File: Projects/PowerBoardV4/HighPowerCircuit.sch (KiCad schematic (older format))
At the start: 27 parts, among them J1 Cell Voltage Sense, J10 5V_INT_PWR_BLK, J11 5V_INT_PWR_BLK, J12 5V_INT_PWR_BLK, J13 5V_INT_PWR_BLK, J14 12V_INT_PWR_BLK, J15 12V_INT_PWR_BLK, J16 12V_INT_PWR_BLK, J17 12V_INT_PWR_BLK, J2 BATT_PWR, J3 12V POWER SUPPLY, J4 5V POWER SUPPLY, J5 BACK_EXT_24V, J7 MC_STACK_1, J8 MC_STACK_2, J9 24V_INT_PWR_BLK, Q1 IRF3205, Q2 IRF3205, Q3 BSS84

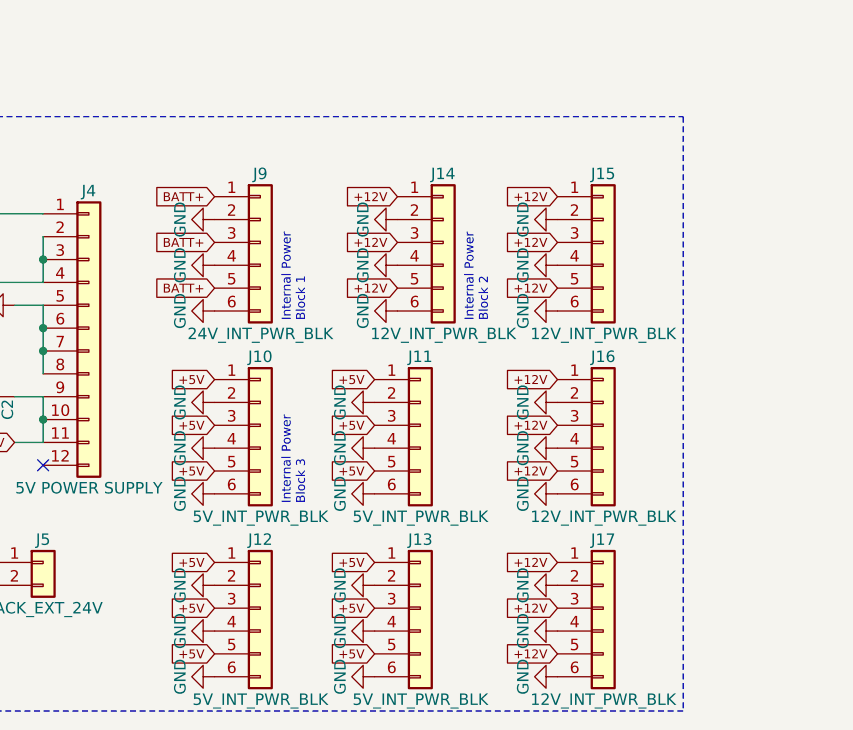
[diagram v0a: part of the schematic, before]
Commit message: Changes complete and ready for review
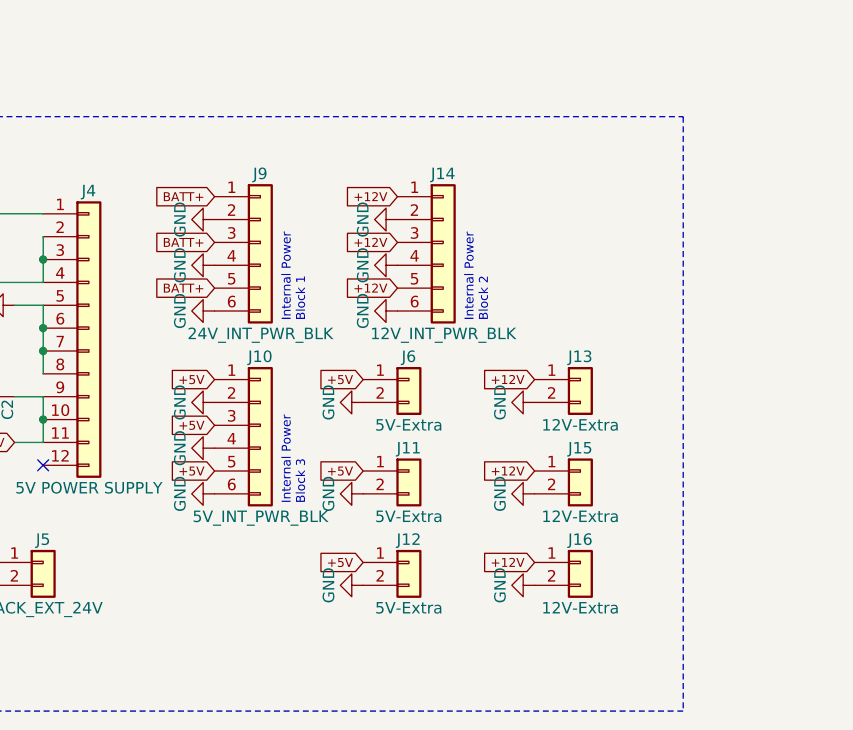
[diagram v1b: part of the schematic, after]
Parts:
- removed J11, J12, J13: 5V_INT_PWR_BLK, Terminal_Blocks:TerminalBlock_Pheonix_PT-3.5mm_6pol, symbol Conn_01x06
- removed J15, J16, J17: 12V_INT_PWR_BLK, USST-footprints:TerminalBlock_Pheonix_PT-5mm_6pol, symbol Conn_01x06
- added J11, J12, J6: 5V-Extra, USST-footprints:Molex_39531_1002, symbol Conn_01x02
- added J13, J15, J16: 12V-Extra, USST-footprints:Molex_39531_1002, symbol Conn_01x02
- J14: footprint USST-footprints:TerminalBlock_Pheonix_PT-5mm_6pol -> Terminal_Blocks:TerminalBlock_Pheonix_PT-3.5mm_6pol
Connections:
- net +12V: now also J13.1 (Pin_1), J15.1 (Pin_1), J16.1 (Pin_1)
- net +5V: now also J11.1 (Pin_1), J12.1 (Pin_1), J6.1 (Pin_1)
- net GND: now also J11.2 (Pin_2), J12.2 (Pin_2), J13.2 (Pin_2), J15.2 (Pin_2), J16.2 (Pin_2), J6.2 (Pin_2)

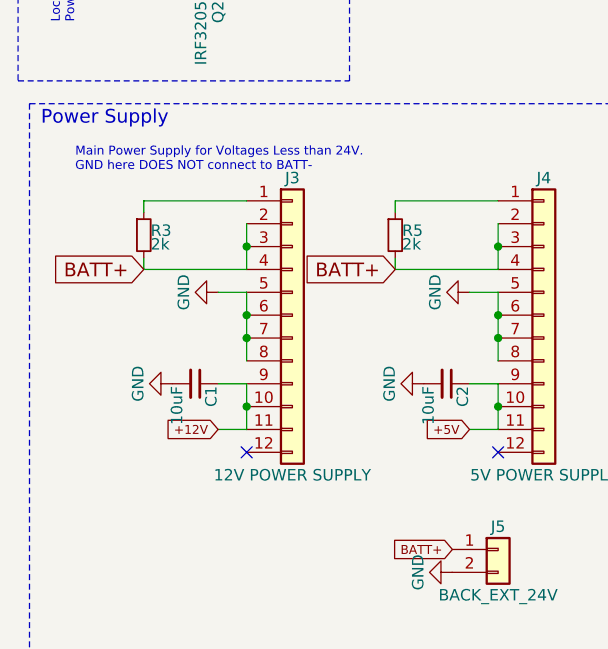
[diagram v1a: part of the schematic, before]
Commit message: Did some more stuff
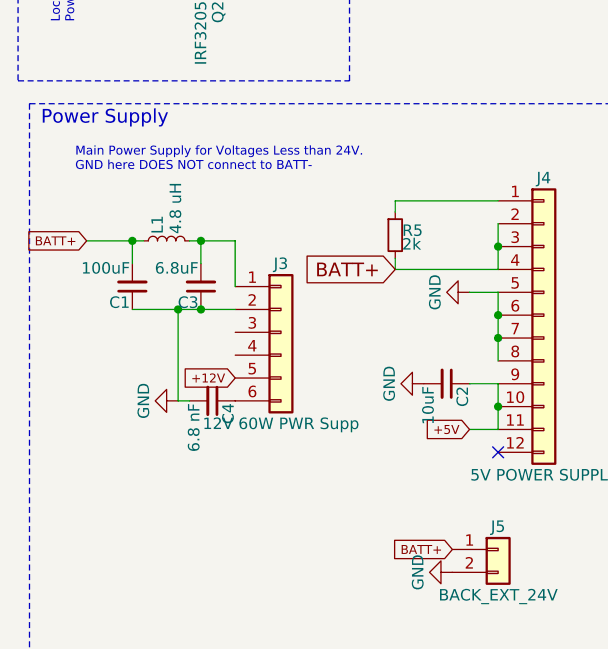
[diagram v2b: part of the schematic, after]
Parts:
- removed J3: 12V POWER SUPPLY, USST-footprints:R-6212P_14-34VDC-12VDC_Converter, symbol Conn_01x12
- removed R3: 2k, Resistors_SMD:R_0603, symbol R_Small
- added C3: 6.8uF, symbol C_Small
- added C4: 6.8 nF, symbol C_Small
- added J3: 12V 60W PWR Supp, symbol Conn_01x06
- added L1: 4.8 uH, symbol L_Small
- C1: value 10uF -> 100uF; footprint Capacitors_ThroughHole:C_Radial_D5_L11_P2.5 -> (none)
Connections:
- net +12V: now also J3.5 (Pin_5); no longer C1.1
- net BATT+: now also C1.2, L1.1
- net GND: now also C1.1, C3.1, C4.2, J3.2 (Pin_2); no longer C1.2
- new net: C3.2, J3.1 (Pin_1), L1.2
- new net: C4.1, J3.6 (Pin_6)
- no-connect marks 2 -> 1
